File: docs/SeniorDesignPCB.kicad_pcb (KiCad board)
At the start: 2 copper layers, 15 parts, among them SW1 RotaryEncoder_Switch, SW2 RotaryEncoder_Switch, U2 STM32F446RETx, U3 RC1602A

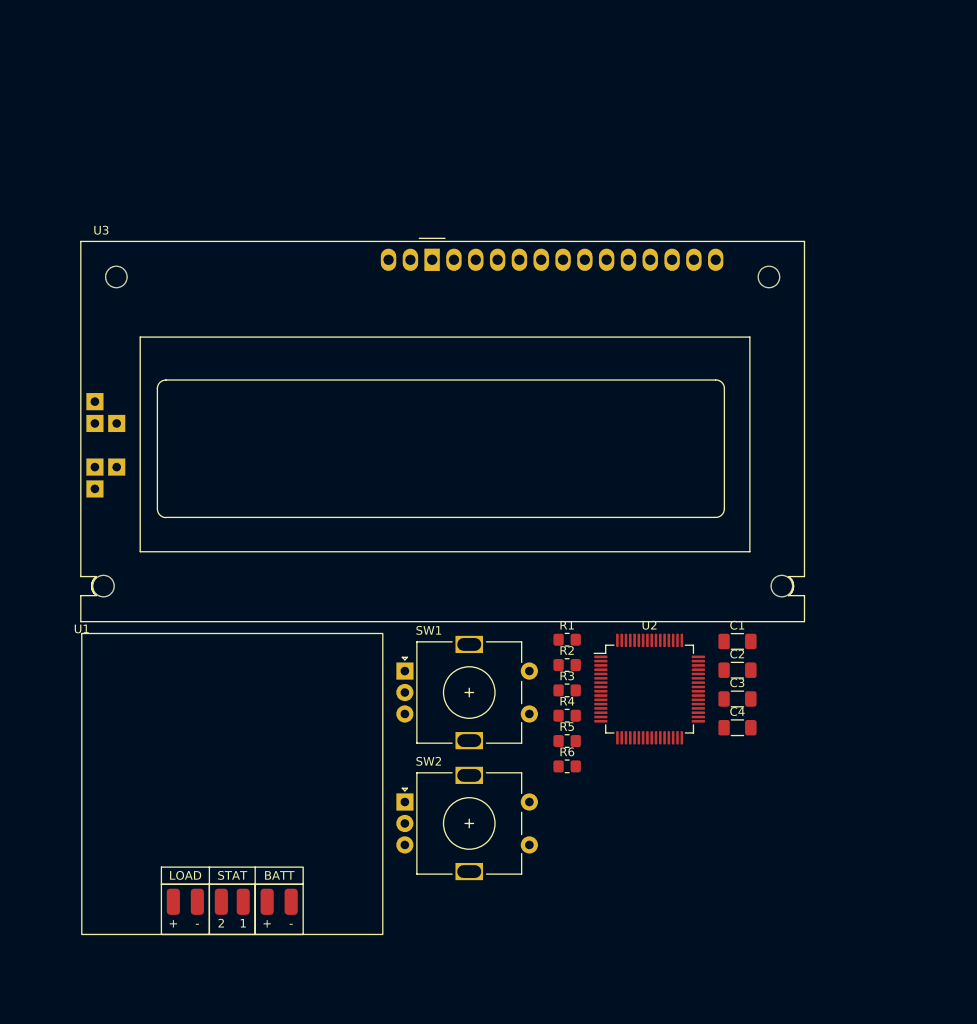
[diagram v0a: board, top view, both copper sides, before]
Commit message: Add files via upload
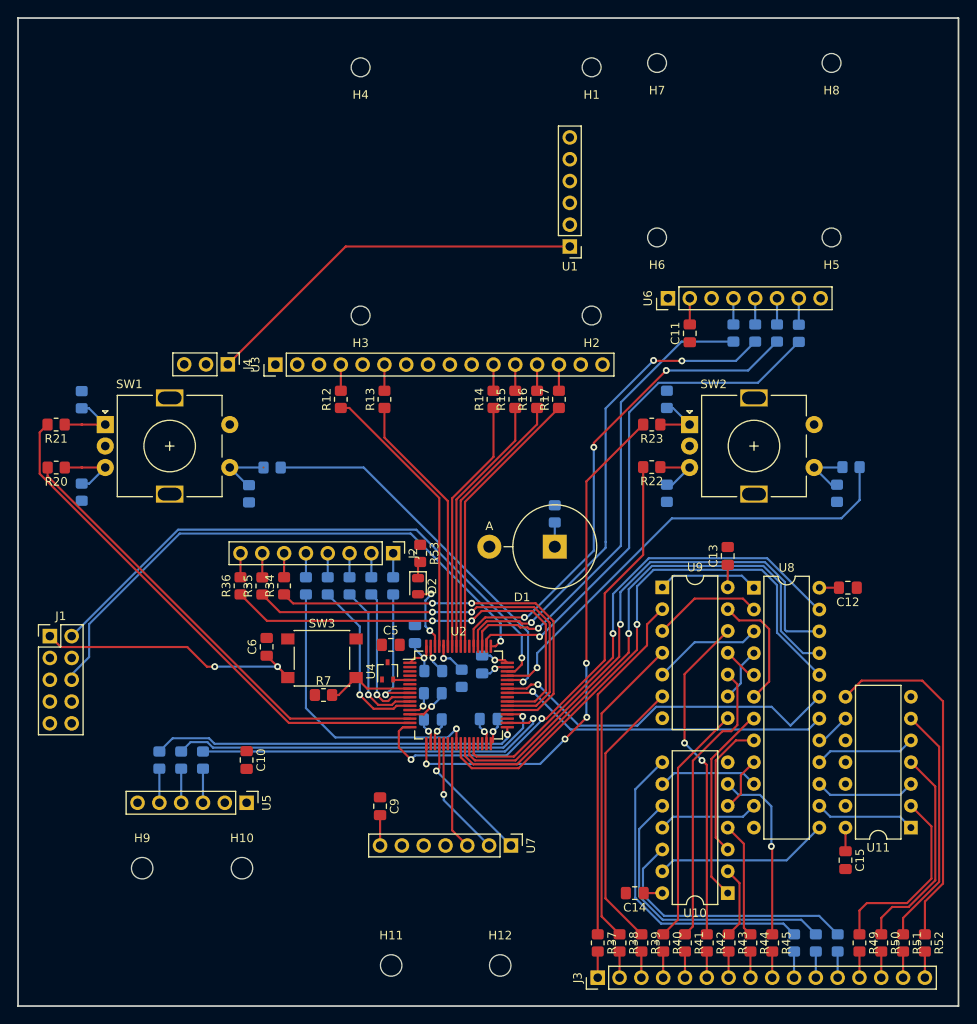
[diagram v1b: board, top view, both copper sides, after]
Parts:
- added C10: 0.1uC, Capacitor_SMD:C_0805_2012Metric_Pad1.18x1.45mm_HandSolder, F.Cu at (126.7, 105.4)
- added C11: 0.1uC, Capacitor_SMD:C_0805_2012Metric_Pad1.18x1.45mm_HandSolder, F.Cu at (178.3, 55.7)
- added C12: 0.1uC, Capacitor_SMD:C_0805_2012Metric_Pad1.18x1.45mm_HandSolder, F.Cu at (196.7, 85.3)
- added C13: 0.1uC, Capacitor_SMD:C_0805_2012Metric_Pad1.18x1.45mm_HandSolder, F.Cu at (182.7, 81.6)
- added C14: 0.1uC, Capacitor_SMD:C_0805_2012Metric_Pad1.18x1.45mm_HandSolder, F.Cu at (171.9, 120.9)
- added C15: 0.1uC, Capacitor_SMD:C_0805_2012Metric_Pad1.18x1.45mm_HandSolder, F.Cu at (196.4, 117.0)
- added C5: 0.1uC, Capacitor_SMD:C_0805_2012Metric_Pad1.18x1.45mm_HandSolder, F.Cu at (143.5, 91.9)
- added C6: 0.1uC, Capacitor_SMD:C_0805_2012Metric_Pad1.18x1.45mm_HandSolder, F.Cu at (129.0, 92.2)
- added C7: 0.1uC, Capacitor_SMD:C_0805_2012Metric_Pad1.18x1.45mm_HandSolder, B.Cu at (146.3, 90.7)
- added C8: 0.1uC, Capacitor_SMD:C_0805_2012Metric_Pad1.18x1.45mm_HandSolder, B.Cu at (148.4, 97.6)
- added C9: 0.1uC, Capacitor_SMD:C_0805_2012Metric_Pad1.18x1.45mm_HandSolder, F.Cu at (142.2, 110.7)
- added D1: LED, Diode_THT:D_5KP_P7.62mm_Vertical_AnodeUp, F.Cu at (162.6, 80.5)
- added D2: LED, Diode_SMD:D_0805_2012Metric, F.Cu at (146.7, 85.1)
- added H1: MountingHole, MountingHole:MountingHole_2.2mm_M2, F.Cu at (166.9, 24.7)
- added H10: MountingHole, MountingHole:MountingHole_2.5mm, F.Cu at (126.2, 118.0)
- added H11: MountingHole, MountingHole:MountingHole_2.5mm, F.Cu at (143.5, 129.3)
- added H12: MountingHole, MountingHole:MountingHole_2.5mm, F.Cu at (156.2, 129.3)
- added H2: MountingHole, MountingHole:MountingHole_2.2mm_M2, F.Cu at (166.9, 53.6)
- added H3: MountingHole, MountingHole:MountingHole_2.2mm_M2, F.Cu at (140.0, 53.6)
- added H4: MountingHole, MountingHole:MountingHole_2.2mm_M2, F.Cu at (140.0, 24.7)
- added H5: MountingHole, MountingHole:MountingHole_2.2mm_M2, F.Cu at (194.8, 44.5)
- added H6: MountingHole, MountingHole:MountingHole_2.2mm_M2, F.Cu at (174.5, 44.5)
- added H7: MountingHole, MountingHole:MountingHole_2.2mm_M2, F.Cu at (174.5, 24.2)
- added H8: MountingHole, MountingHole:MountingHole_2.2mm_M2, F.Cu at (194.8, 24.2)
- added H9: MountingHole, MountingHole:MountingHole_2.5mm, F.Cu at (114.5, 118.0)
- added J1: Conn_02x05_Odd_Even, Connector_PinHeader_2.54mm:PinHeader_2x05_P2.54mm_Vertical, F.Cu at (103.8, 90.9)
- added J2: Conn_01x08_Pin, Connector_PinHeader_2.54mm:PinHeader_1x08_P2.54mm_Vertical, F.Cu at (143.8, 81.3)
- added J3: Conn_01x16_Pin, Connector_PinHeader_2.54mm:PinHeader_1x16_P2.54mm_Vertical, F.Cu at (167.6, 130.7)
- added J4: Conn_01x03_Pin, Connector_PinHeader_2.54mm:PinHeader_1x03_P2.54mm_Vertical, F.Cu at (124.5, 59.3)
- added R10: 30R, Resistor_SMD:R_0805_2012Metric_Pad1.20x1.40mm_HandSolder, B.Cu at (119.1, 105.4)
- added R11: 30R, Resistor_SMD:R_0805_2012Metric_Pad1.20x1.40mm_HandSolder, B.Cu at (116.5, 105.4)
- added R12: 20R, Resistor_SMD:R_0805_2012Metric_Pad1.20x1.40mm_HandSolder, F.Cu at (137.7, 63.4)
- added R13: 20R, Resistor_SMD:R_0805_2012Metric_Pad1.20x1.40mm_HandSolder, F.Cu at (142.7, 63.4)
- added R14: 20R, Resistor_SMD:R_0805_2012Metric_Pad1.20x1.40mm_HandSolder, F.Cu at (155.4, 63.4)
- added R15: 20R, Resistor_SMD:R_0805_2012Metric_Pad1.20x1.40mm_HandSolder, F.Cu at (158.0, 63.4)
- added R16: 20R, Resistor_SMD:R_0805_2012Metric_Pad1.20x1.40mm_HandSolder, F.Cu at (160.5, 63.4)
- added R17: 20R, Resistor_SMD:R_0805_2012Metric_Pad1.20x1.40mm_HandSolder, F.Cu at (163.1, 63.4)
- added R18: 20R, Resistor_SMD:R_0805_2012Metric_Pad1.20x1.40mm_HandSolder, B.Cu at (197.1, 71.2)
- added R19: 20R, Resistor_SMD:R_0805_2012Metric_Pad1.20x1.40mm_HandSolder, B.Cu at (129.7, 71.3)
- added R20: 20R, Resistor_SMD:R_0805_2012Metric_Pad1.20x1.40mm_HandSolder, F.Cu at (104.5, 71.3)
- added R21: 20R, Resistor_SMD:R_0805_2012Metric_Pad1.20x1.40mm_HandSolder, F.Cu at (104.5, 66.3)
- added R22: 20R, Resistor_SMD:R_0805_2012Metric_Pad1.20x1.40mm_HandSolder, F.Cu at (173.9, 71.2)
- added R23: 20R, Resistor_SMD:R_0805_2012Metric_Pad1.20x1.40mm_HandSolder, F.Cu at (173.9, 66.3)
- added R24: 20R, Resistor_SMD:R_0805_2012Metric_Pad1.20x1.40mm_HandSolder, B.Cu at (183.4, 55.6)
- added R25: 20R, Resistor_SMD:R_0805_2012Metric_Pad1.20x1.40mm_HandSolder, B.Cu at (185.9, 55.6)
- added R26: 20R, Resistor_SMD:R_0805_2012Metric_Pad1.20x1.40mm_HandSolder, B.Cu at (188.5, 55.6)
- added R27: 20R, Resistor_SMD:R_0805_2012Metric_Pad1.20x1.40mm_HandSolder, B.Cu at (191.0, 55.7)
- added R28: 100R, Resistor_SMD:R_0805_2012Metric_Pad1.20x1.40mm_HandSolder, B.Cu at (162.6, 76.7)
- added R29: 20R, Resistor_SMD:R_0805_2012Metric_Pad1.20x1.40mm_HandSolder, B.Cu at (143.8, 85.1)
- added R30: 20R, Resistor_SMD:R_0805_2012Metric_Pad1.20x1.40mm_HandSolder, B.Cu at (141.2, 85.1)
- added R31: 20R, Resistor_SMD:R_0805_2012Metric_Pad1.20x1.40mm_HandSolder, B.Cu at (138.7, 85.1)
- added R32: 20R, Resistor_SMD:R_0805_2012Metric_Pad1.20x1.40mm_HandSolder, B.Cu at (136.1, 85.1)
- added R33: 20R, Resistor_SMD:R_0805_2012Metric_Pad1.20x1.40mm_HandSolder, B.Cu at (133.6, 85.1)
- added R34: 20R, Resistor_SMD:R_0805_2012Metric_Pad1.20x1.40mm_HandSolder, F.Cu at (131.1, 85.1)
- added R35: 20R, Resistor_SMD:R_0805_2012Metric_Pad1.20x1.40mm_HandSolder, F.Cu at (128.5, 85.1)
- added R36: 20R, Resistor_SMD:R_0805_2012Metric_Pad1.20x1.40mm_HandSolder, F.Cu at (126.0, 85.1)
- added R37: 20R, Resistor_SMD:R_0805_2012Metric_Pad1.20x1.40mm_HandSolder, F.Cu at (167.6, 126.7)
- added R38: 20R, Resistor_SMD:R_0805_2012Metric_Pad1.20x1.40mm_HandSolder, F.Cu at (170.1, 126.7)
- added R39: 20R, Resistor_SMD:R_0805_2012Metric_Pad1.20x1.40mm_HandSolder, F.Cu at (172.7, 126.7)
- added R40: 20R, Resistor_SMD:R_0805_2012Metric_Pad1.20x1.40mm_HandSolder, F.Cu at (175.2, 126.7)
- added R41: 20R, Resistor_SMD:R_0805_2012Metric_Pad1.20x1.40mm_HandSolder, F.Cu at (177.7, 126.7)
- added R42: 20R, Resistor_SMD:R_0805_2012Metric_Pad1.20x1.40mm_HandSolder, F.Cu at (180.3, 126.7)
- added R43: 20R, Resistor_SMD:R_0805_2012Metric_Pad1.20x1.40mm_HandSolder, F.Cu at (182.8, 126.7)
- added R44: 20R, Resistor_SMD:R_0805_2012Metric_Pad1.20x1.40mm_HandSolder, F.Cu at (185.4, 126.7)
- added R45: 20R, Resistor_SMD:R_0805_2012Metric_Pad1.20x1.40mm_HandSolder, F.Cu at (187.9, 126.7)
- added R46: 20R, Resistor_SMD:R_0805_2012Metric_Pad1.20x1.40mm_HandSolder, B.Cu at (190.5, 126.7)
- added R47: 20R, Resistor_SMD:R_0805_2012Metric_Pad1.20x1.40mm_HandSolder, B.Cu at (193.0, 126.7)
- added R48: 20R, Resistor_SMD:R_0805_2012Metric_Pad1.20x1.40mm_HandSolder, B.Cu at (195.5, 126.7)
- added R49: 20R, Resistor_SMD:R_0805_2012Metric_Pad1.20x1.40mm_HandSolder, F.Cu at (198.1, 126.7)
- added R50: 20R, Resistor_SMD:R_0805_2012Metric_Pad1.20x1.40mm_HandSolder, F.Cu at (200.6, 126.7)
- added R51: 20R, Resistor_SMD:R_0805_2012Metric_Pad1.20x1.40mm_HandSolder, F.Cu at (203.1, 126.7)
- added R52: 20R, Resistor_SMD:R_0805_2012Metric_Pad1.20x1.40mm_HandSolder, F.Cu at (205.7, 126.7)
- added R53: 100R, Resistor_SMD:R_0805_2012Metric_Pad1.20x1.40mm_HandSolder, F.Cu at (146.9, 81.3)
- added R7: 100k, Resistor_SMD:R_0805_2012Metric_Pad1.20x1.40mm_HandSolder, F.Cu at (135.7, 97.8)
- added R8: 100k, Resistor_SMD:R_0805_2012Metric_Pad1.20x1.40mm_HandSolder, B.Cu at (151.7, 95.8)
- added R9: 30R, Resistor_SMD:R_0805_2012Metric_Pad1.20x1.40mm_HandSolder, B.Cu at (121.6, 105.4)
- added SW3: SW_Push, Button_Switch_SMD:SW_Push_1P1T_NO_6x6mm_H9.5mm, F.Cu at (135.5, 93.5)
- added U10: 74LS04, Package_DIP:DIP-14_W7.62mm, F.Cu at (182.7, 120.9)
- added U11: 74LS04, Package_DIP:DIP-14_W7.62mm, F.Cu at (204.1, 113.2)
- added U4: MAX7375AXR805, Package_TO_SOT_SMD:SOT-323_SC-70, F.Cu at (143.1, 95.0)
- added U5: ~, Connector_PinHeader_2.54mm:PinHeader_1x06_P2.54mm_Vertical, F.Cu at (126.7, 110.3)
- added U6: ~, Connector_PinHeader_2.54mm:PinHeader_1x08_P2.54mm_Vertical, F.Cu at (175.8, 51.6)
- added U7: ~, Connector_PinHeader_2.54mm:PinHeader_1x07_P2.54mm_Vertical, F.Cu at (157.5, 115.3)
- added U8: 74HC154, Package_DIP:DIP-24_W7.62mm, F.Cu at (185.8, 85.3)
- added U9: 74LS04, Package_DIP:DIP-14_W7.62mm, F.Cu at (175.1, 85.3)
- C1, C2, C3, C4: footprint Capacitor_SMD:C_1206_3216Metric_Pad1.33x1.80mm_HandSolder -> Capacitor_SMD:C_0805_2012Metric_Pad1.18x1.45mm_HandSolder; moved to B.Cu
- R1, R2, R3, R4, R5, R6: moved to B.Cu
- U1: footprint SeniorDesignFPLibrary:PCB_BatteryManagement -> Connector_PinHeader_2.54mm:PinHeader_1x06_P2.54mm_Vertical
- U3: footprint Display:RC1602A -> Connector_PinHeader_2.54mm:PinHeader_1x16_P2.54mm_Vertical
- moved U1 72.5 mm to (164.3, 45.6), turned to 180 degrees
- moved R2 64.4 mm to (107.5, 63.4), turned to 90 degrees
- moved R1 59.1 mm to (107.5, 74.2), turned to -90 degrees
- moved SW2 55.1 mm to (178.3, 66.3)
- moved SW1 45.2 mm to (110.2, 66.3)
- moved R6 44.7 mm to (195.5, 74.3), turned to 90 degrees
- moved R3 43.6 mm to (127.0, 74.4), turned to 90 degrees
- moved R5 41.5 mm to (175.6, 63.4), turned to 90 degrees
- moved C1 36.6 mm to (148.4, 100.6)
- moved C4 36.0 mm to (148.4, 95.0), turned to 180 degrees
- moved C3 30.0 mm to (154.1, 94.2), turned to 90 degrees
- moved C2 29.5 mm to (154.9, 100.6)
- moved R4 28.4 mm to (175.6, 74.3), turned to -90 degrees
- moved U2 22.3 mm to (151.4, 97.8)
- moved U3 22.0 mm to (130.0, 59.3), turned to 90 degrees
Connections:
- C1 pad 2: Net-(U1-Load+) -> +3.3V
- C2 pad 2: Net-(U1-Load+) -> +3.3V
- C3 pad 2: Net-(U1-Load+) -> +3.3V
- C4 pad 2: Net-(U1-Load+) -> +3.3V
- R1 pad 1: +3.3V -> Net-(R1-Pad1)
- R1 pad 2: Net-(U2-PA13) -> +3.3V
- R2 pad 1: +3.3V -> Net-(R2-Pad1)
- R2 pad 2: Net-(U2-PA14) -> +3.3V
- R3 pad 1: Net-(U2-PA0) -> +3.3V
- R3 pad 2: +3.3V -> Net-(R19-Pad2)
- R4 pad 1: Net-(U2-PA1) -> Net-(R22-Pad1)
- R5 pad 1: Net-(U2-PA6) -> Net-(R23-Pad1)
- R6 pad 1: Net-(U2-PA7) -> +3.3V
- R6 pad 2: +3.3V -> Net-(R18-Pad2)
- SW1 pad A: Net-(U2-PA1) -> Net-(R2-Pad1)
- SW1 pad B: Net-(U2-PA0) -> Net-(R1-Pad1)
- SW1 pad S1: Net-(U2-PA13) -> Net-(R19-Pad2)
- SW2 pad A: Net-(U2-PA7) -> Net-(R23-Pad1)
- SW2 pad B: Net-(U2-PA6) -> Net-(R22-Pad1)
- SW2 pad S1: Net-(U2-PA14) -> Net-(R18-Pad2)
- U1 pad 1: unconnected-(U1-VBus-Pad1) -> /VDD_BAT
- U1 pad 2: unconnected-(U1-D+-Pad2) -> GND
- U2 pad 1: unconnected-(U2-VBAT-Pad1) -> +3.3V
- U2 pad 10: unconnected-(U2-PC2-Pad10) -> /PC2
- U2 pad 11: unconnected-(U2-PC3-Pad11) -> /PC3
- U2 pad 12: unconnected-(U2-VSSA-Pad12) -> GND
- U2 pad 13: unconnected-(U2-VDDA-Pad13) -> +3.3V
- U2 pad 14: Net-(U2-PA0) -> /PA0
- U2 pad 15: Net-(U2-PA1) -> /PA1
- U2 pad 16: unconnected-(U2-PA2-Pad16) -> /PA2
- U2 pad 17: unconnected-(U2-PA3-Pad17) -> /PA3
- U2 pad 19: Net-(U1-Load+) -> +3.3V
- U2 pad 20: unconnected-(U2-PA4-Pad20) -> /PA4
- U2 pad 21: unconnected-(U2-PA5-Pad21) -> /PA5
- U2 pad 22: Net-(U2-PA6) -> unconnected-(U2-PA6-Pad22)
- U2 pad 23: Net-(U2-PA7) -> /PA7
- U2 pad 24: unconnected-(U2-PC4-Pad24) -> /PC4
- U2 pad 25: unconnected-(U2-PC5-Pad25) -> /PC5
- U2 pad 26: unconnected-(U2-PB0-Pad26) -> /PB0
- U2 pad 27: Net-(U2-PB1) -> /PB1
- U2 pad 28: Net-(U2-PB2) -> /PB2
- U2 pad 32: Net-(U1-Load+) -> +3.3V
- U2 pad 33: unconnected-(U2-PB12-Pad33) -> /PB12
- U2 pad 34: unconnected-(U2-PB13-Pad34) -> /PB13
- U2 pad 36: unconnected-(U2-PB15-Pad36) -> /PB15
- U2 pad 37: unconnected-(U2-PC6-Pad37) -> /PC6
- U2 pad 38: unconnected-(U2-PC7-Pad38) -> /PC7
- U2 pad 39: unconnected-(U2-PC8-Pad39) -> /PC8
- U2 pad 41: unconnected-(U2-PA8-Pad41) -> /PA8
- U2 pad 42: unconnected-(U2-PA9-Pad42) -> /PA9
- U2 pad 44: unconnected-(U2-PA11-Pad44) -> /PA11
- U2 pad 45: unconnected-(U2-PA12-Pad45) -> /PA12
- U2 pad 46: Net-(U2-PA13) -> /SWDIO
- U2 pad 48: Net-(U1-Load+) -> +3.3V
- U2 pad 49: Net-(U2-PA14) -> /SWCLK
- U2 pad 5: unconnected-(U2-PH0-Pad5) -> /OSC_IN
- U2 pad 50: unconnected-(U2-PA15-Pad50) -> /PA15
- U2 pad 51: unconnected-(U2-PC10-Pad51) -> /PC10
- U2 pad 52: unconnected-(U2-PC11-Pad52) -> /PC11
- U2 pad 53: unconnected-(U2-PC12-Pad53) -> /PC12
- U2 pad 55: Net-(U2-PB3) -> /PB3
- U2 pad 56: Net-(U2-PB4) -> /PB4
- U2 pad 57: Net-(U2-PB5) -> /PB5
- U2 pad 58: Net-(U2-PB6) -> /PB6
- U2 pad 59: unconnected-(U2-PB7-Pad59) -> /PB7
- U2 pad 60: unconnected-(U2-BOOT0-Pad60) -> /BOOT0
- U2 pad 61: unconnected-(U2-PB8-Pad61) -> /PB8
- U2 pad 62: unconnected-(U2-PB9-Pad62) -> /DB_LED
- U2 pad 64: Net-(U1-Load+) -> +3.3V
- U2 pad 7: unconnected-(U2-NRST-Pad7) -> /NRST
- U2 pad 8: unconnected-(U2-PC0-Pad8) -> /PC0
- U2 pad 9: unconnected-(U2-PC1-Pad9) -> /PC1
- U3 pad 11: Net-(U2-PB3) -> Net-(U3-DB4)
- U3 pad 12: Net-(U2-PB4) -> Net-(U3-DB5)
- U3 pad 13: Net-(U2-PB5) -> Net-(U3-DB6)
- U3 pad 14: Net-(U2-PB6) -> Net-(U3-DB7)
- U3 pad 4: Net-(U2-PB1) -> Net-(U3-RS)
- U3 pad 6: Net-(U2-PB2) -> Net-(U3-E)
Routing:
- net /SWDIO: track 0.00 -> 68.1 mm, vias 0 -> 1
- net /SWCLK: track 0.00 -> 67.4 mm, vias 0 -> 1
- net /PC5: track 0.00 -> 66.1 mm, vias 0 -> 1
- net /PB0: track 0.00 -> 64.5 mm, vias 0 -> 1
- net /PB1: track 0.00 -> 62.9 mm, vias 0 -> 1
- net /PA1: track 0.00 -> 61.2 mm
- net /PA15: track 0.00 -> 61.0 mm, vias 0 -> 1
- net /PA3: track 0.00 -> 60.5 mm, vias 0 -> 4
- net /PC12: track 0.00 -> 58.6 mm, vias 0 -> 3
- net /PC11: track 0.00 -> 58.2 mm, vias 0 -> 3
- net /PB2: track 0.00 -> 58.0 mm, vias 0 -> 1
- net /PA2: track 0.00 -> 57.2 mm, vias 0 -> 2
- net /PC10: track 0.00 -> 55.1 mm, vias 0 -> 1
- net /PA0: track 0.00 -> 54.9 mm
- net /PA12: track 0.00 -> 54.5 mm, vias 0 -> 1
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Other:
- board outline added: 109.5 x 115.1 mm
